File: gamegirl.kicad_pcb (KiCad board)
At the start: 2 copper layers, 58 parts, among them J1 Conn_01x07_Socket, J2 Conn_01x14_Socket, J3 Conn_01x04_Socket, SW1 EN, SW10 select, SW12 SS12D07VG4 087, SW2 up, SW3 down, SW4 left, SW5 right, SW6 A, SW7 B, SW8 BOOT, SW9 start, U1 ESP32-WROOM-32, U2 AP2112K-3.3, U3 CH340N_C2977777

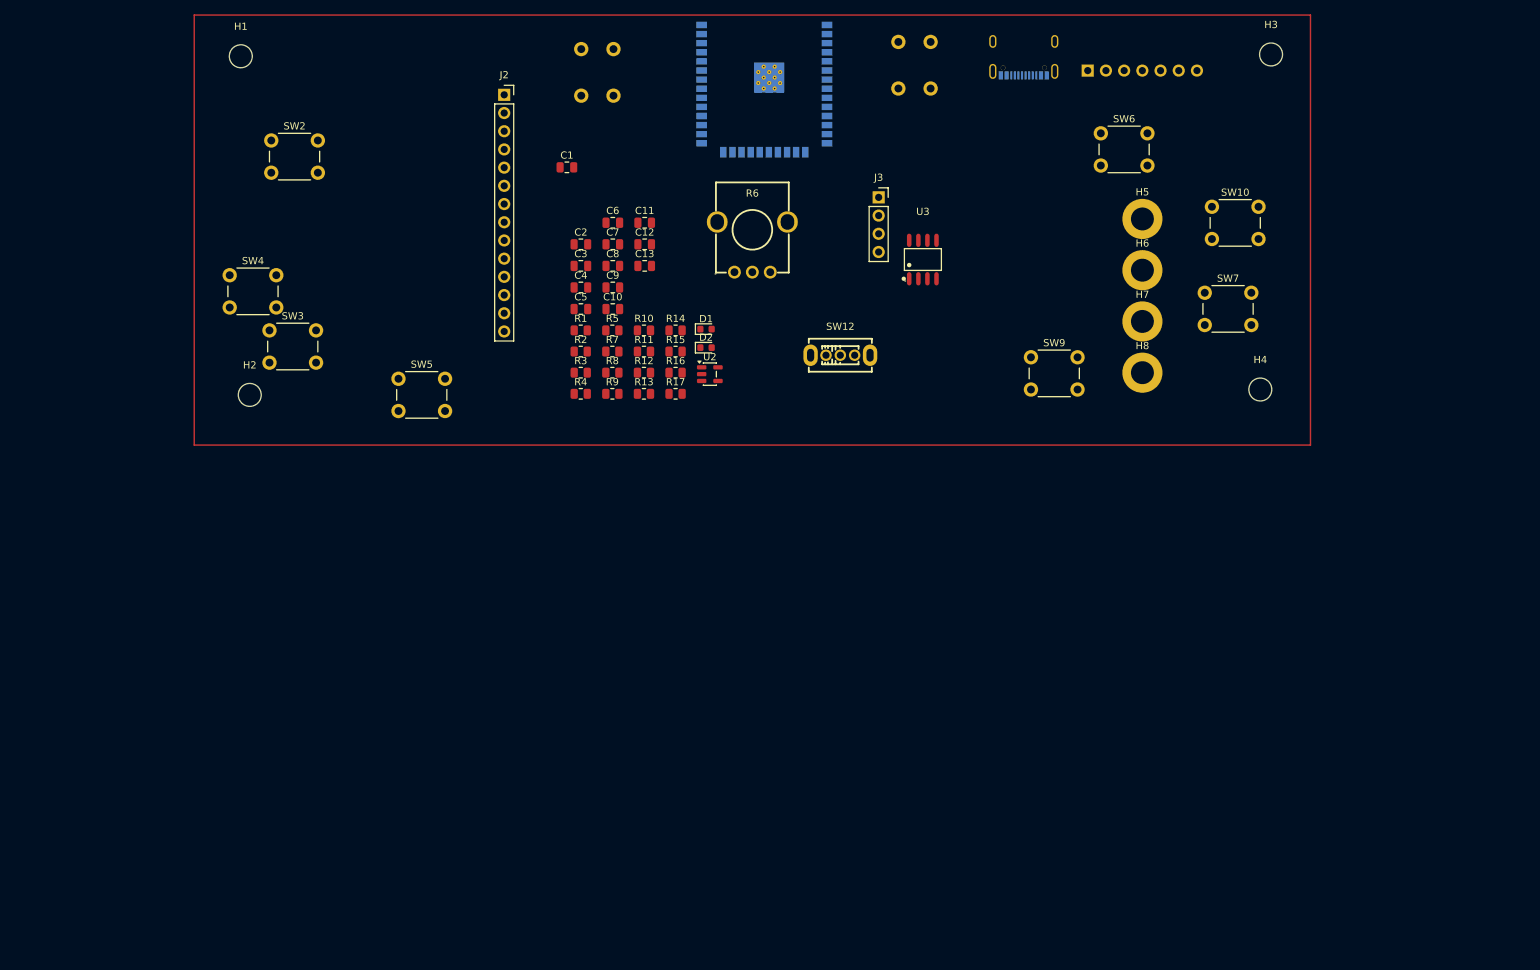
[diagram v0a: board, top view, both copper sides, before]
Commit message: why is this display so big
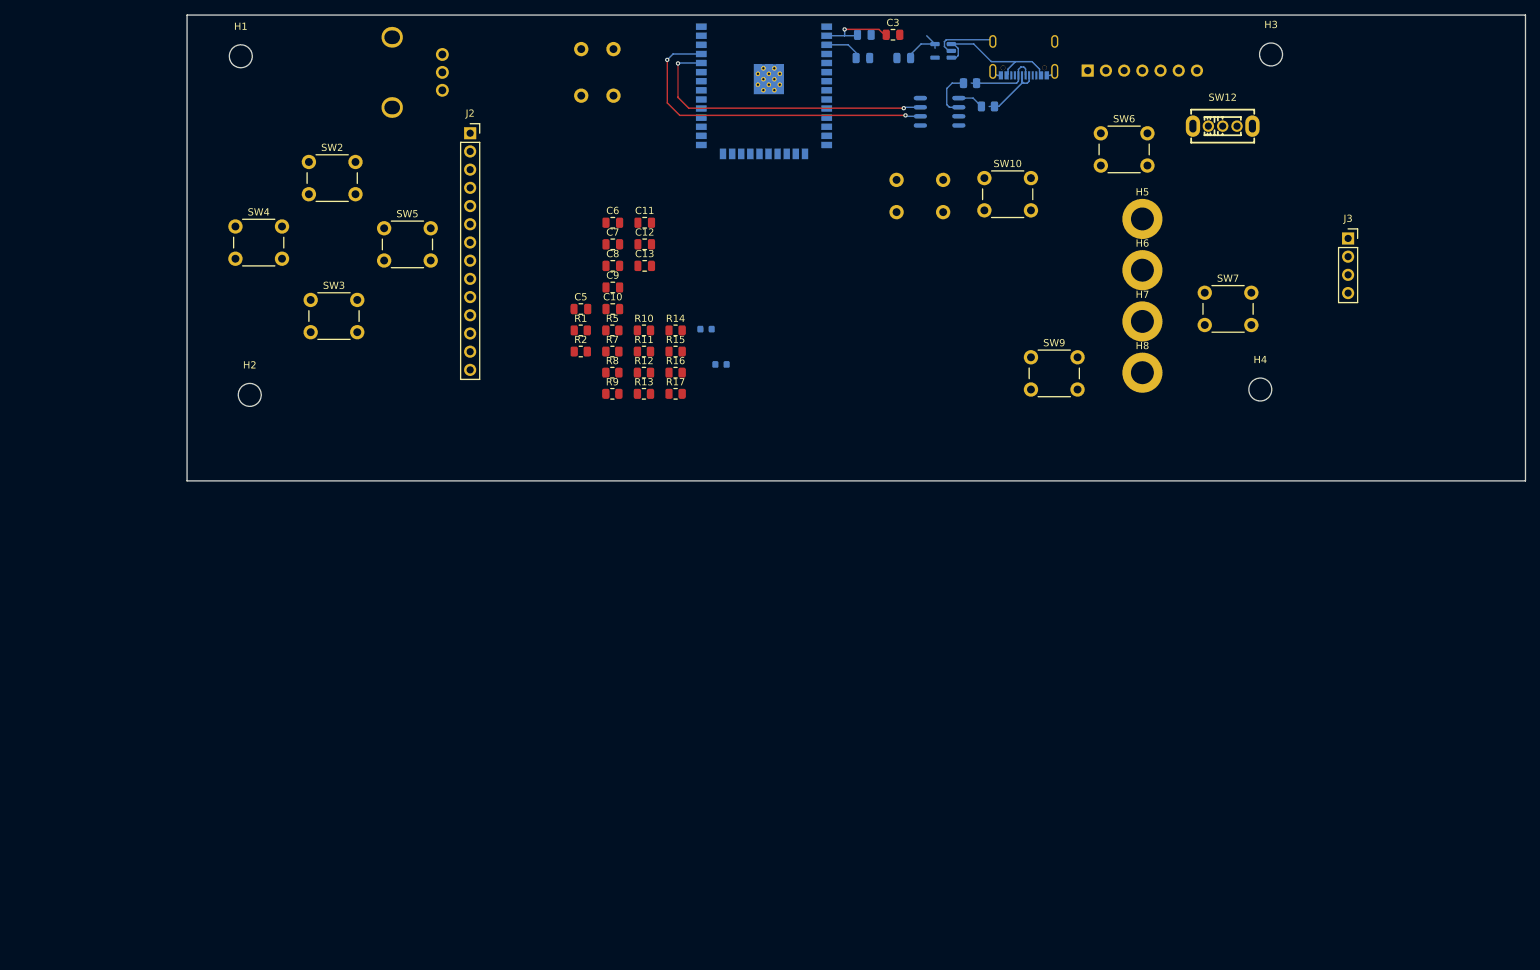
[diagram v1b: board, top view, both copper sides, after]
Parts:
- C1, C2, C4, D1, D2, R3, R4, R6, U2, U3: moved to B.Cu
- moved R4 69.5 mm to (178.0, 45.5), turned to 180 degrees
- moved R3 67.9 mm to (180.5, 48.8), turned to 180 degrees
- moved J3 65.8 mm to (230.8, 67.2)
- moved SW12 62.2 mm to (213.2, 51.5)
- moved U2 55.6 mm to (174.2, 41.0), turned to 180 degrees
- moved C3 54.2 mm to (167.2, 38.8)
- moved C4 53.0 mm to (163.2, 38.8), turned to 180 degrees
- moved R6 52.7 mm to (100.9, 44.0), turned to -90 degrees
- moved C1 49.4 mm to (168.8, 42.0)
- moved C2 47.2 mm to (163.1, 42.0)
- moved SW10 32.0 mm to (180.0, 58.8)
- moved SW5 21.1 mm to (96.2, 65.8)
- moved U3 20.7 mm to (173.8, 49.5), turned to -90 degrees
- moved SW1 17.9 mm to (167.8, 63.5), turned to 0 degrees
- moved J2 7.16 mm to (108.2, 52.5)
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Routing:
- net /tx: track 0.00 -> 47.2 mm, vias 0 -> 2
- net /rx: track 0.00 -> 42.5 mm, vias 0 -> 2
- net VBUS: track 0.00 -> 20.8 mm
- net +3V3: track 0.00 -> 17.7 mm, vias 0 -> 1
- net GND: track 0.00 -> 11.6 mm, vias 0 -> 12
- net usb dm: track 0.00 -> 10.5 mm
- net usb dp: track 0.00 -> 9.88 mm
- net Net-(U3-UD-): track 0.00 -> 6.73 mm
- net Net-(U1-EN): track 0.00 -> 4.55 mm
- net Net-(U3-UD+): track 0.00 -> 3.64 mm
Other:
- board outline added: 186.8 x 65 mm

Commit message: rough layout
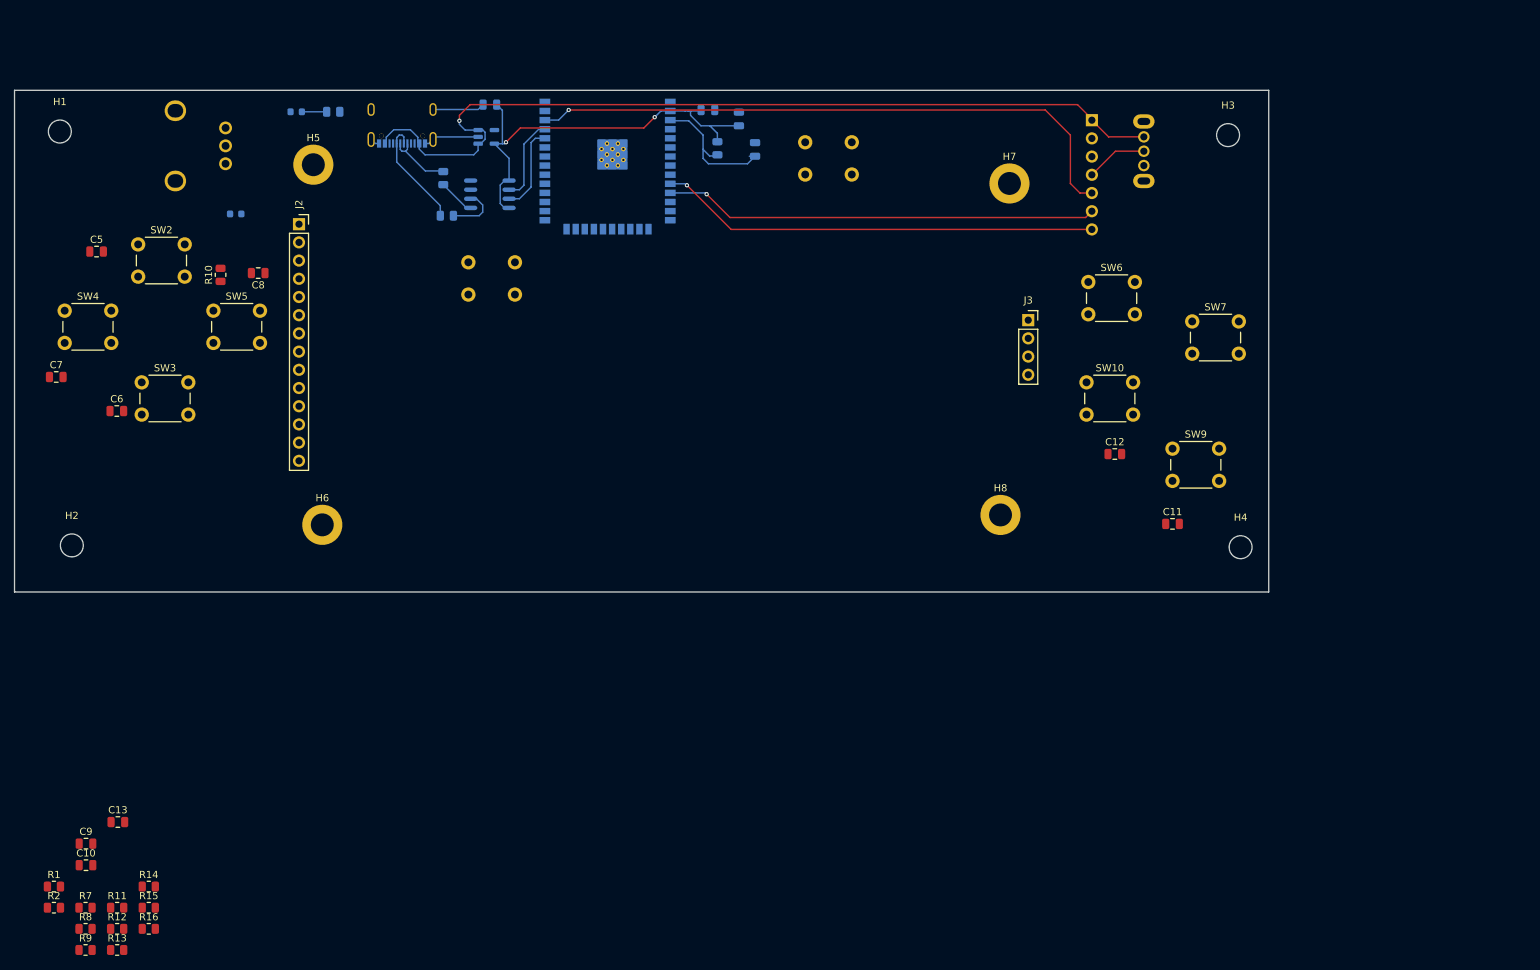
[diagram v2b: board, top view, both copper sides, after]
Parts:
- C3, R17, R5, SW12: moved to B.Cu
- moved H6 119.8 mm to (87.6, 107.1)
- moved H5 115.9 mm to (86.4, 56.9)
- moved C10 106.9 mm to (54.6, 154.6)
- moved C9 106.9 mm to (54.6, 151.6)
- moved R11 106.9 mm to (59.0, 160.6)
- moved R15 106.9 mm to (63.4, 160.6)
- moved R2 106.9 mm to (50.2, 160.6)
- moved R7 106.9 mm to (54.6, 160.6)
- moved C13 106.9 mm to (59.1, 148.6)
- moved R1 106.9 mm to (50.2, 157.6)
- moved R12 106.9 mm to (59.0, 163.5)
- moved R13 106.9 mm to (59.0, 166.4)
- moved R14 106.9 mm to (63.4, 157.6)
- moved R16 106.9 mm to (63.4, 163.5)
- moved R8 106.9 mm to (54.6, 163.5)
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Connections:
- J2 pad 1: unconnected-(J2-Pin_1-Pad1) -> +3V3
- J2 pad 10: /GPIO2 -> unconnected-(J2-Pin_10-Pad10)
- J2 pad 11: /GPIO4 -> unconnected-(J2-Pin_11-Pad11)
- J2 pad 12: /GPIO5 -> unconnected-(J2-Pin_12-Pad12)
- J2 pad 13: GND -> unconnected-(J2-Pin_13-Pad13)
- J2 pad 14: +3V3 -> unconnected-(J2-Pin_14-Pad14)
- J2 pad 2: unconnected-(J2-Pin_2-Pad2) -> GND
- J2 pad 3: unconnected-(J2-Pin_3-Pad3) -> /GPIO5
- J2 pad 4: unconnected-(J2-Pin_4-Pad4) -> /GPIO4
- J2 pad 5: unconnected-(J2-Pin_5-Pad5) -> /GPIO2
- J2 pad 6: /GPIO19 -> /GPIO23
- J2 pad 7: /LCD_BRIGHT -> /GPIO18
- J2 pad 8: /GPIO18 -> /LCD_BRIGHT
- J2 pad 9: /GPIO23 -> /GPIO19
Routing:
- net VBUS: track 20.8 -> 123.3 mm, vias 0 -> 1
- net /GPIO22: track 0.00 -> 85.7 mm, vias 0 -> 1
- net /GPIO25: track 0.00 -> 61.5 mm, vias 0 -> 1
- net /GPIO26: track 0.00 -> 60.6 mm, vias 0 -> 1
- net +3V3: track 17.7 -> 58.7 mm, vias 1 -> 2
- net /tx: track 47.2 -> 11.9 mm, vias 2 -> 0
- net /rx: track 42.5 -> 12.1 mm, vias 2 -> 0
- net Net-(U1-EN): track 4.55 -> 19.9 mm
- net /GAIN: track 0.00 -> 8.61 mm
- net GND: track 11.6 -> 16.7 mm
- net usb dm: track 10.5 -> 15.6 mm
- net Net-(D1-A): track 0.00 -> 3.46 mm
- net Net-(U3-UD+): track 3.64 -> 5.17 mm
- net usb dp: track 9.88 -> 8.60 mm
- net Net-(U3-UD-): track 6.73 -> 7.33 mm
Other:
- board size 186.8 x 65 mm -> 175 x 70 mm
